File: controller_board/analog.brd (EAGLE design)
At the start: 121 x 115.3 mm, 111 parts

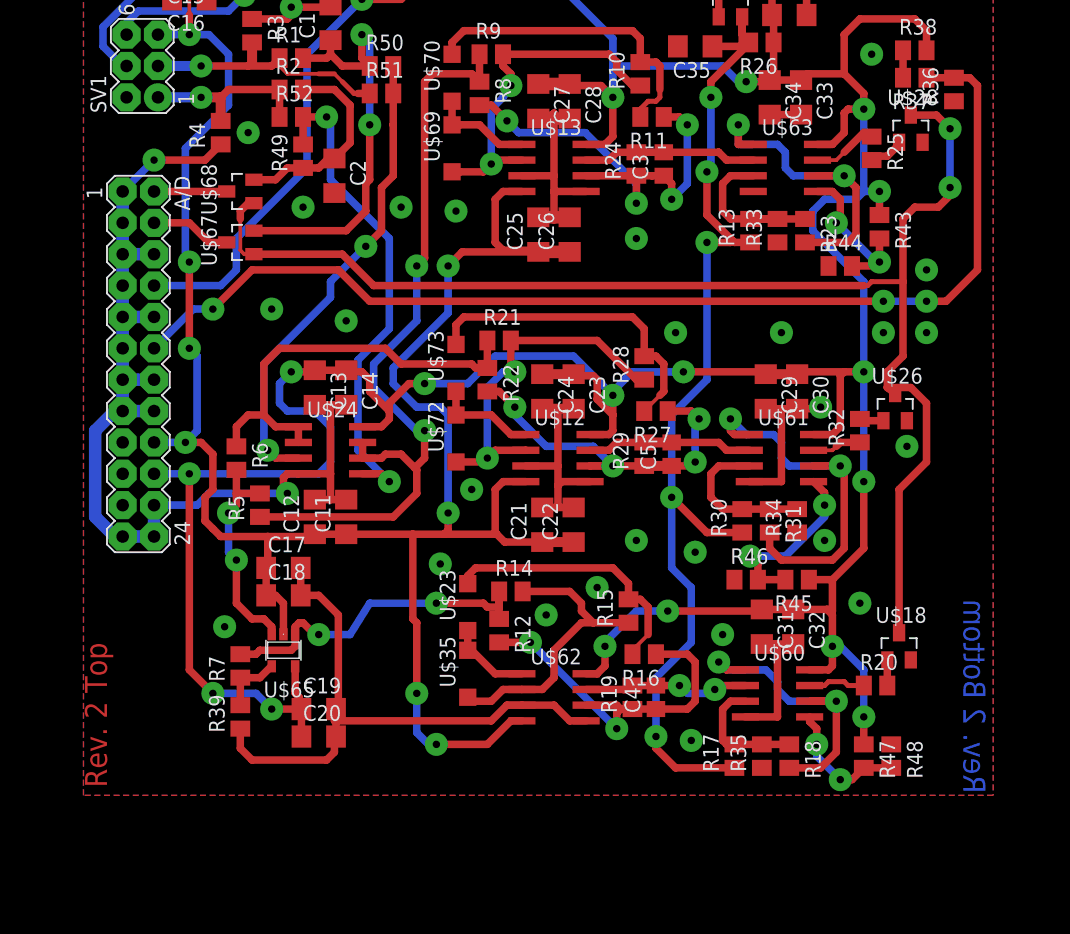
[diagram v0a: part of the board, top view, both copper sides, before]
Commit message: Pull commit
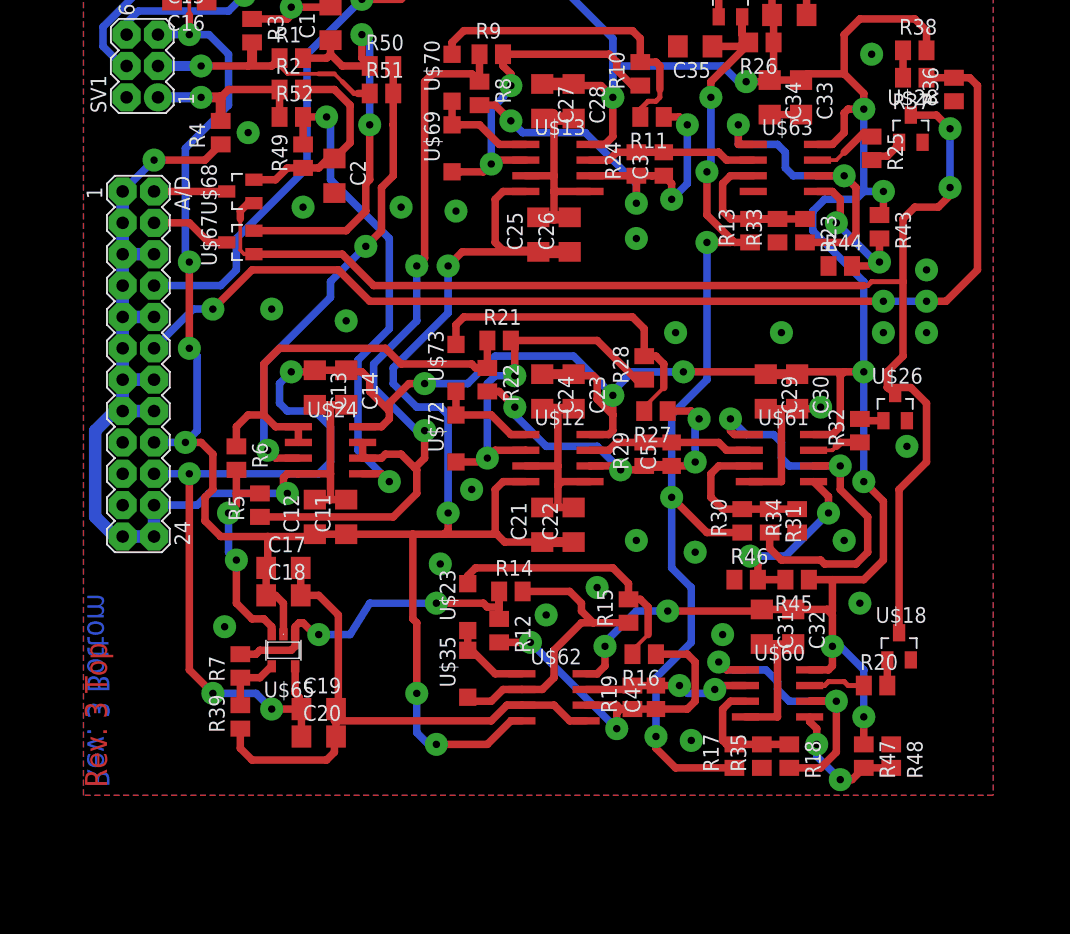
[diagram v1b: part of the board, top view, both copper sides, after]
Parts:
- moved C27 0.32 mm to (37.1, 63.8)
- moved C28 0.32 mm to (39.7, 63.8)
- moved U$13 0.32 mm to (38.4, 58.4)
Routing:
- net N$30: track 30.9 -> 34.0 mm
- net +15V: track 349.2 -> 352.2 mm
- net N$24: track 28.1 -> 29.8 mm
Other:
- board text added: "Rev. 3 Bottom"
- board text added: "Rev. 3 Top"
- board text removed: "Rev. 2 Bottom"
- board text removed: "Rev. 2 Top"
